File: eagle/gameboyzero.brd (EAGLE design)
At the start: 71 x 88 mm, 22 parts

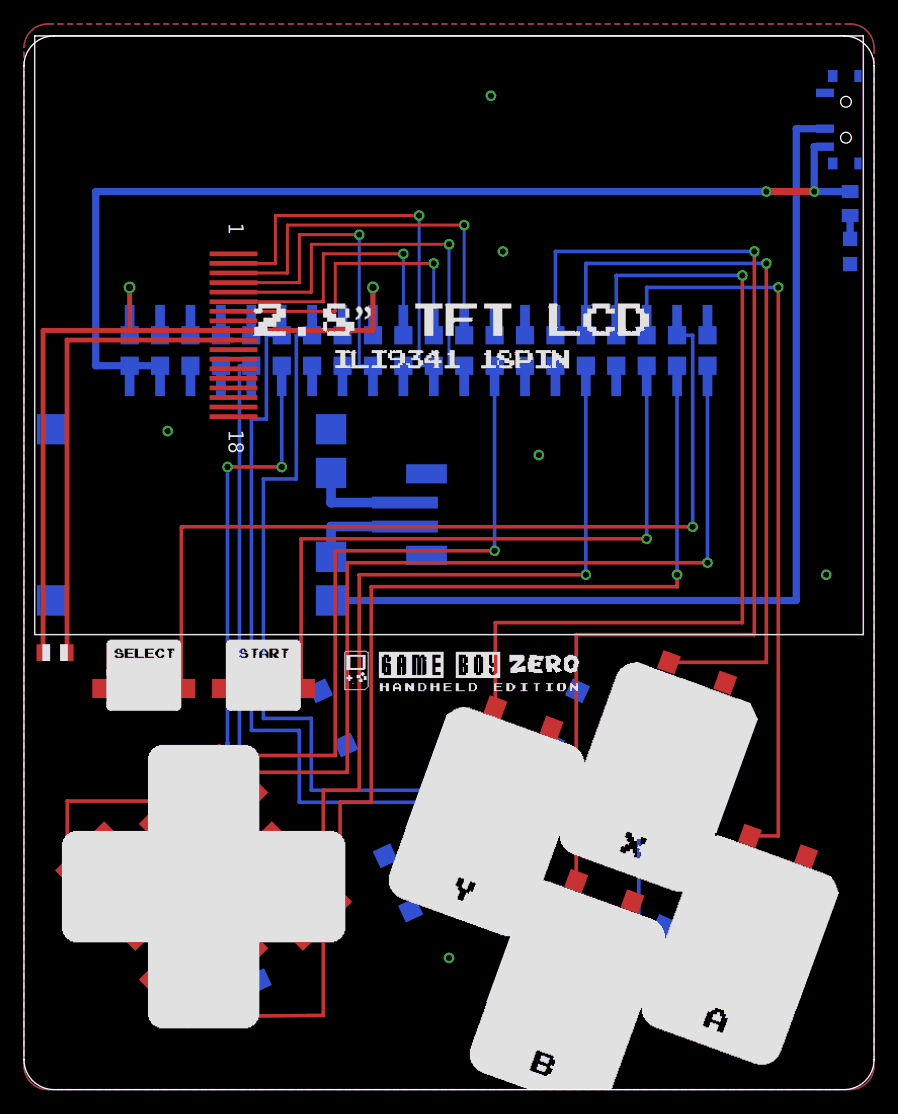
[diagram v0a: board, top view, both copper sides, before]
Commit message: updates
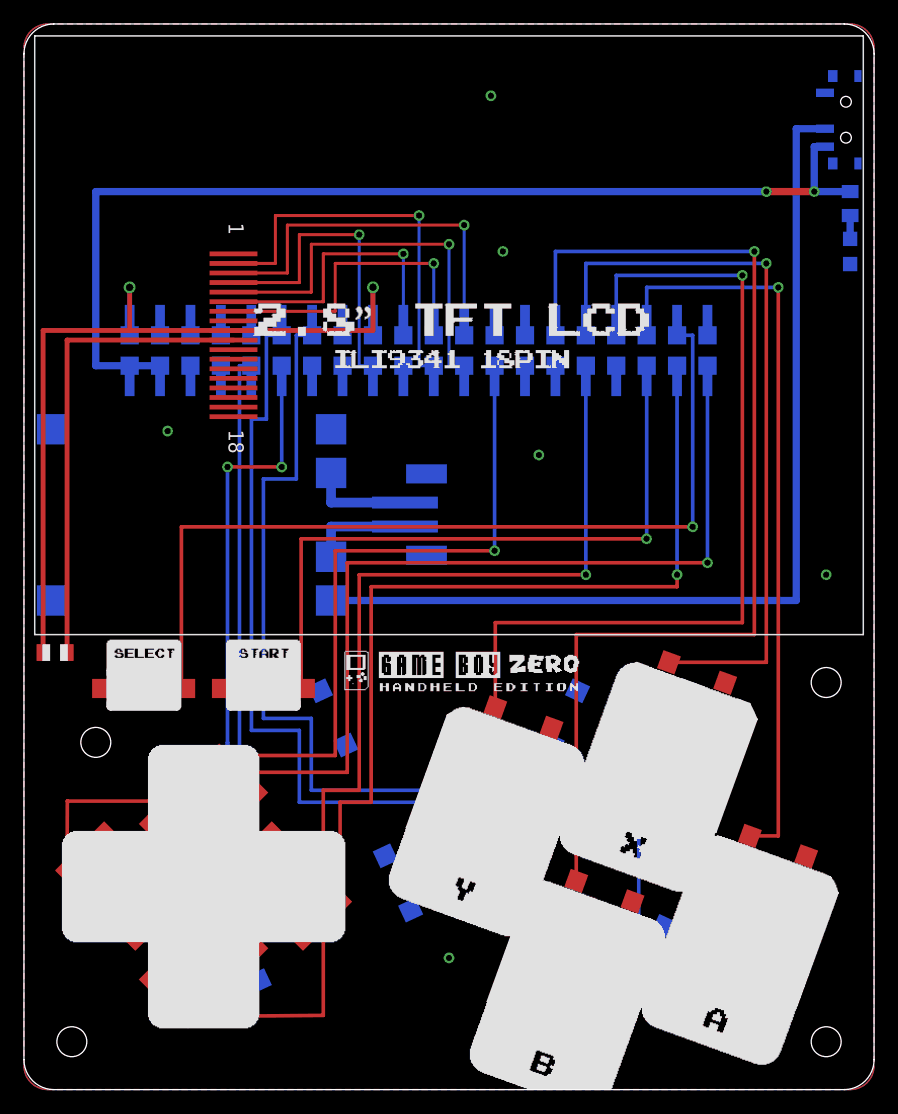
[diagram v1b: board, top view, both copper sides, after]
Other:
- board size 71 x 88 mm -> 71 x 89 mm
